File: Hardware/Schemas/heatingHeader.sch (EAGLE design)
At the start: 26 parts, among them IC1 DS1820

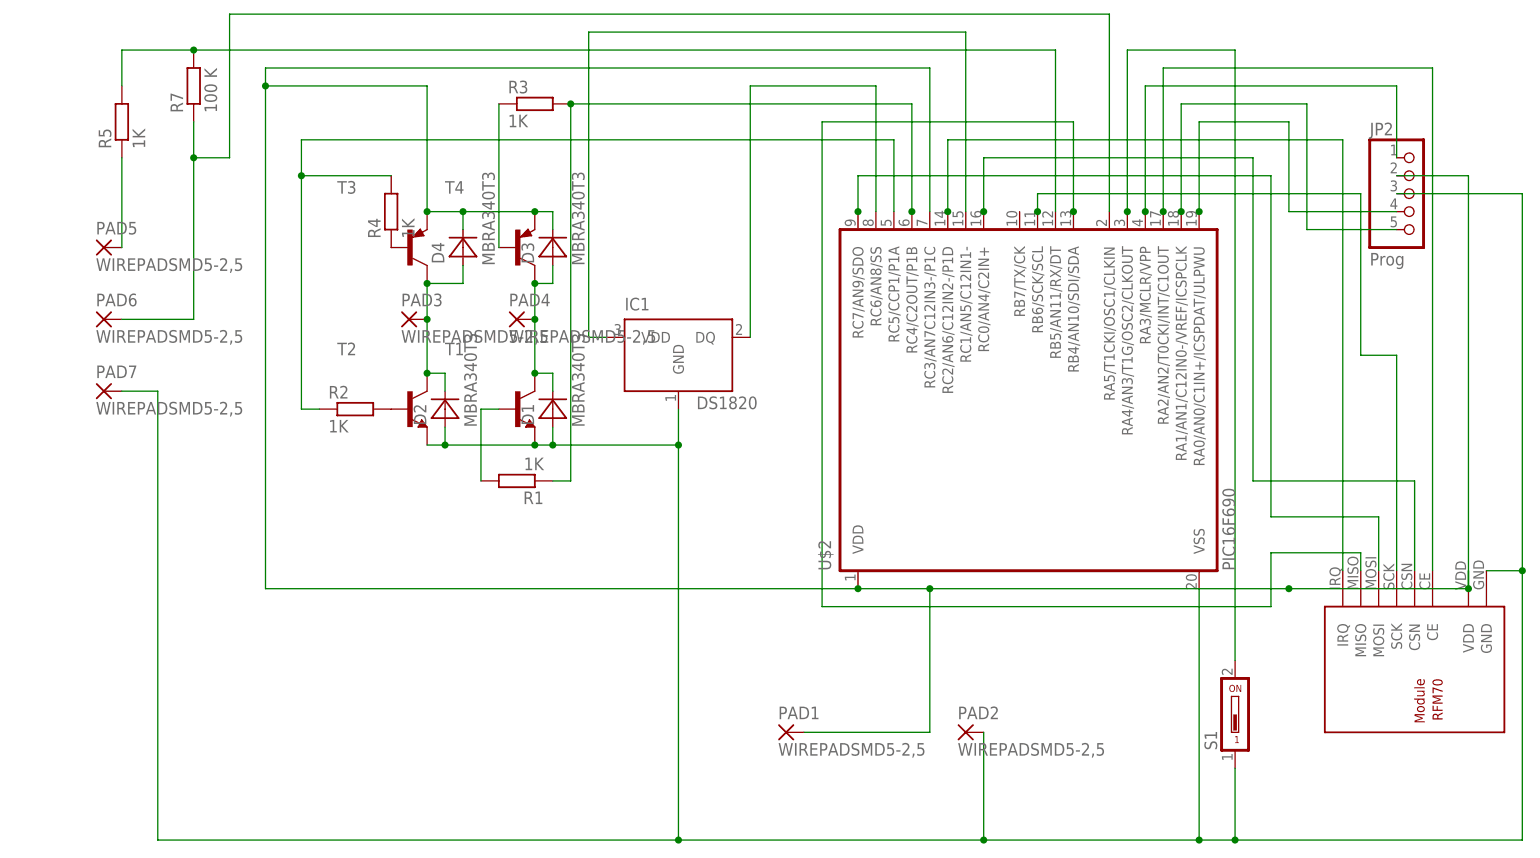
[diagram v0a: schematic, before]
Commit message: a
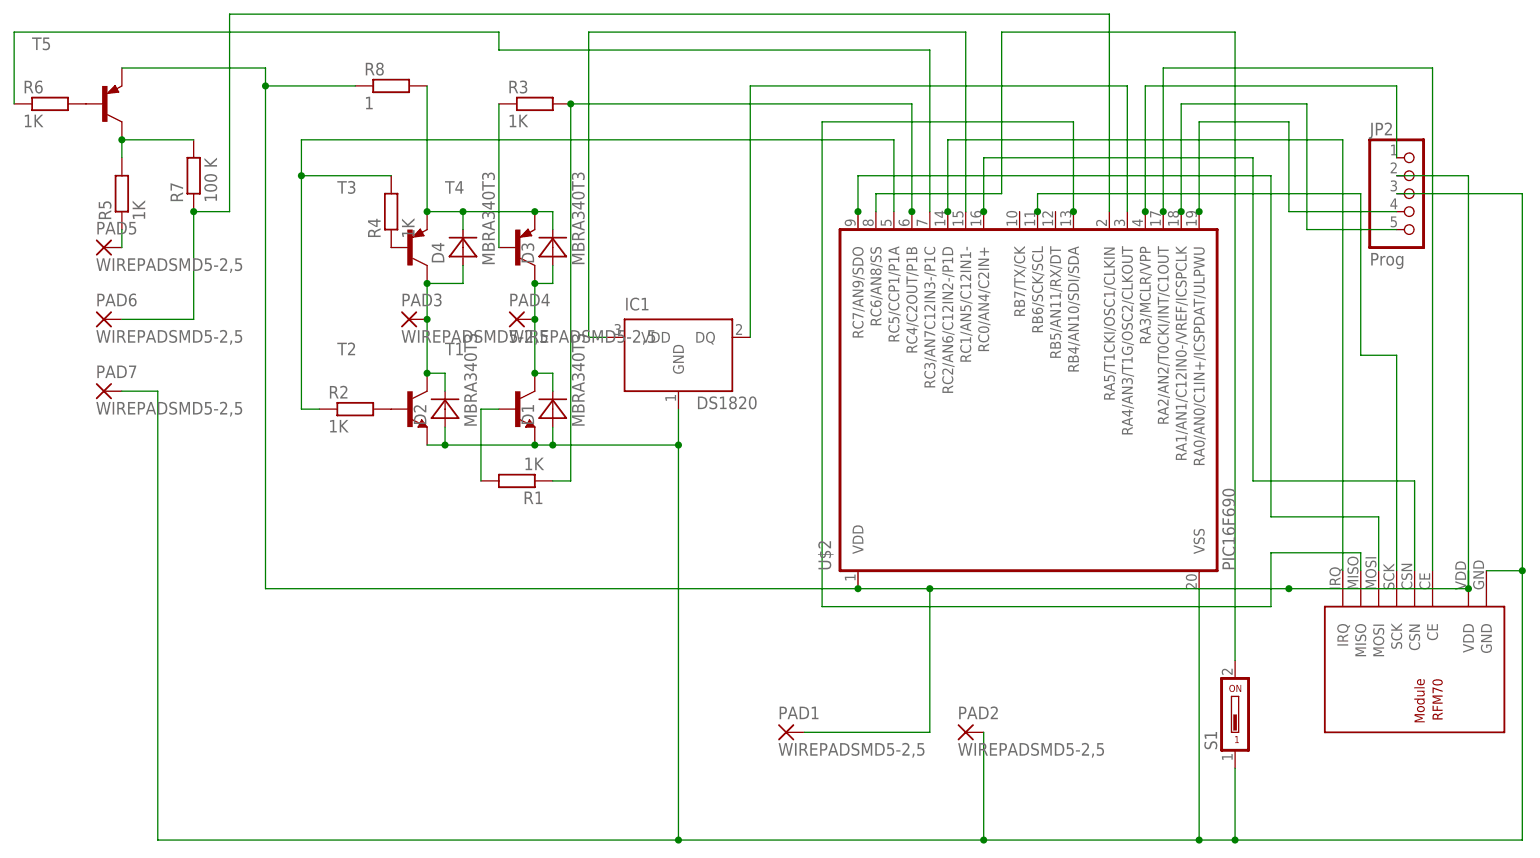
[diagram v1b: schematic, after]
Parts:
- added R6: 1K, resistor:R-EU_R1206
- added R8: 1, resistor:R-EU_R0805W
- added T5: (no value), transistor:BC807-16-PNP-SOT23-BEC
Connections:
- new net N$11: R6.2, T5.B
- new net N$12: R6.1, U$2.RC3/AN7C12IN3-/P1C
- new net N$15: D3.C, D4.C, R8.2, T3.E, T4.E
- net N$1: now also U$2.RA4/AN3/T1G/OSC2/CLKOUT; no longer U$2.RC6/AN8/SS
- net N$10: now also U$2.RC6/AN8/SS; no longer U$2.RA4/AN3/T1G/OSC2/CLKOUT
- net N$2: now also R8.1, T5.E; no longer D3.C, D4.C, T3.E, T4.E, U$2.RC3/AN7C12IN3-/P1C
- net N$28: now also T5.C; no longer U$2.RB5/AN11/RX/DT
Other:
- moved on the sheet: R5, R7
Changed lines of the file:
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@@
 <part name="R7" library="resistor" deviceset="R-EU_" device="R1206" value="100 K"/>
 <part name="S1" library="switch-dil" deviceset="SD4-01" device=""/>
+<part name="T5" library="transistor" deviceset="*-PNP-" device="SOT23-BEC" technology="BC807-16"/>
+<part name="R6" library="resistor" deviceset="R-EU_" device="R1206" value="1K"/>
+<part name="R8" library="resistor" deviceset="R-EU_" device="R0805W" value="1"/>
 </parts>
 <sheets>
@@
 <instance part="PAD4" gate="G$1" x="35.56" y="104.14"/>
 <instance part="PAD5" gate="G$1" x="-22.86" y="114.3"/>
-<instance part="R5" gate="G$1" x="-20.32" y="132.08" rot="R90"/>
+<instance part="R5" gate="G$1" x="-20.32" y="121.92" rot="R90"/>
 <instance part="PAD6" gate="G$1" x="-22.86" y="104.14"/>
 <instance part="PAD7" gate="G$1" x="-22.86" y="93.98"/>
-<instance part="R7" gate="G$1" x="-10.16" y="137.16" rot="R90"/>
+<instance part="R7" gate="G$1" x="-10.16" y="124.46" rot="R90"/>
 <instance part="S1" gate="1" x="137.16" y="48.26"/>
+<instance part="T5" gate="G$1" x="-22.86" y="134.62"/>
+<instance part="R6" gate="G$1" x="-30.48" y="134.62"/>
+<instance part="R8" gate="G$1" x="17.78" y="137.16"/>
 </instances>
 <busses>
@@
 <segment>
 <pinref part="R5" gate="G$1" pin="2"/>
-<wire x1="111.76" y1="142.24" x2="-10.16" y2="142.24" width="0.1524" layer="91"/>
-<wire x1="-10.16" y1="142.24" x2="-20.32" y2="142.24" width="0.1524" layer="91"/>
-<wire x1="-20.32" y1="142.24" x2="-20.32" y2="137.16" width="0.1524" layer="91"/>
-<pinref part="U$2" gate="G$1" pin="RB5/AN11/RX/DT"/>
-<wire x1="111.76" y1="119.38" x2="111.76" y2="142.24" width="0.1524" layer="91"/>
+<wire x1="-10.16" y1="129.54" x2="-20.32" y2="129.54" width="0.1524" layer="91"/>
+<wire x1="-20.32" y1="129.54" x2="-20.32" y2="127" width="0.1524" layer="91"/>
 <pinref part="R7" gate="G$1" pin="2"/>
-<junction x="-10.16" y="142.24"/>
+<pinref part="T5" gate="G$1" pin="C"/>
+<junction x="-20.32" y="129.54"/>
 </segment>
 </net>
@@
 <pinref part="IC1" gate="G$1" pin="DQ"/>
 <wire x1="68.58" y1="101.6" x2="68.58" y2="137.16" width="0.1524" layer="91"/>
-<pinref part="U$2" gate="G$1" pin="RC6/AN8/SS"/>
-<wire x1="68.58" y1="137.16" x2="86.36" y2="137.16" width="0.1524" layer="91"/>
-<wire x1="86.36" y1="137.16" x2="86.36" y2="119.38" width="0.1524" layer="91"/>
+<pinref part="U$2" gate="G$1" pin="RA4/AN3/T1G/OSC2/CLKOUT"/>
+<wire x1="121.92" y1="119.38" x2="121.92" y2="137.16" width="0.1524" layer="91"/>
+<wire x1="121.92" y1="137.16" x2="68.58" y2="137.16" width="0.1524" layer="91"/>
 </segment>
 </net>
@@
 <pinref part="R5" gate="G$1" pin="1"/>
 <pinref part="PAD5" gate="G$1" pin="P"/>
-<wire x1="-20.32" y1="127" x2="-20.32" y2="114.3" width="0.1524" layer="91"/>
+<wire x1="-20.32" y1="116.84" x2="-20.32" y2="114.3" width="0.1524" layer="91"/>
 </segment>
 </net>
 <net name="N$2" class="0">
 <segment>
-<pinref part="T4" gate="G$1" pin="E"/>
-<pinref part="D3" gate="G$1" pin="C"/>
-<wire x1="40.64" y1="116.84" x2="40.64" y2="119.38" width="0.1524" layer="91"/>
-<wire x1="40.64" y1="119.38" x2="38.1" y2="119.38" width="0.1524" layer="91"/>
-<junction x="38.1" y="119.38"/>
-<wire x1="27.94" y1="119.38" x2="38.1" y2="119.38" width="0.1524" layer="91"/>
-<pinref part="D4" gate="G$1" pin="C"/>
-<wire x1="27.94" y1="116.84" x2="27.94" y2="119.38" width="0.1524" layer="91"/>
-<junction x="27.94" y="119.38"/>
-<pinref part="T3" gate="G$1" pin="E"/>
-<wire x1="22.86" y1="119.38" x2="27.94" y2="119.38" width="0.1524" layer="91"/>
-<junction x="22.86" y="119.38"/>
-<wire x1="22.86" y1="137.16" x2="22.86" y2="119.38" width="0.1524" layer="91"/>
-<wire x1="22.86" y1="137.16" x2="0" y2="137.16" width="0.1524" layer="91"/>
+<wire x1="0" y1="139.7" x2="0" y2="137.16" width="0.1524" layer="91"/>
+<pinref part="U$2" gate="G$1" pin="VDD"/>
 <wire x1="0" y1="137.16" x2="0" y2="66.04" width="0.1524" layer="91"/>
-<pinref part="U$2" gate="G$1" pin="RC3/AN7C12IN3-/P1C"/>
-<wire x1="93.98" y1="119.38" x2="93.98" y2="139.7" width="0.1524" layer="91"/>
-<wire x1="93.98" y1="139.7" x2="0" y2="139.7" width="0.1524" layer="91"/>
-<wire x1="0" y1="139.7" x2="0" y2="137.16" width="0.1524" layer="91"/>
-<junction x="0" y="137.16"/>
-<pinref part="U$2" gate="G$1" pin="VDD"/>
 <wire x1="83.82" y1="66.04" x2="93.98" y2="66.04" width="0.1524" layer="91"/>
 <pinref part="U$1" gate="G$1" pin="VDD"/>
@@
 <wire x1="0" y1="66.04" x2="83.82" y2="66.04" width="0.1524" layer="91"/>
 <junction x="83.82" y="66.04"/>
+<pinref part="T5" gate="G$1" pin="E"/>
+<wire x1="-20.32" y1="139.7" x2="0" y2="139.7" width="0.1524" layer="91"/>
+<pinref part="R8" gate="G$1" pin="1"/>
+<wire x1="0" y1="137.16" x2="12.7" y2="137.16" width="0.1524" layer="91"/>
+<junction x="0" y="137.16"/>
 </segment>
 </net>
@@
 <wire x1="119.38" y1="119.38" x2="119.38" y2="147.32" width="0.1524" layer="91"/>
 <wire x1="119.38" y1="147.32" x2="-5.08" y2="147.32" width="0.1524" layer="91"/>
-<wire x1="-5.08" y1="147.32" x2="-5.08" y2="127" width="0.1524" layer="91"/>
+<wire x1="-5.08" y1="147.32" x2="-5.08" y2="119.38" width="0.1524" layer="91"/>
 <pinref part="R7" gate="G$1" pin="1"/>
-<wire x1="-10.16" y1="132.08" x2="-10.16" y2="127" width="0.1524" layer="91"/>
 <pinref part="PAD6" gate="G$1" pin="P"/>
-<wire x1="-10.16" y1="127" x2="-10.16" y2="104.14" width="0.1524" layer="91"/>
+<wire x1="-10.16" y1="119.38" x2="-10.16" y2="104.14" width="0.1524" layer="91"/>
 <wire x1="-10.16" y1="104.14" x2="-20.32" y2="104.14" width="0.1524" layer="91"/>
-<wire x1="-5.08" y1="127" x2="-10.16" y2="127" width="0.1524" layer="91"/>
-<junction x="-10.16" y="127"/>
+<wire x1="-5.08" y1="119.38" x2="-10.16" y2="119.38" width="0.1524" layer="91"/>
+<junction x="-10.16" y="119.38"/>
 </segment>
 </net>
@@
 <segment>
 <pinref part="S1" gate="1" pin="2"/>
-<wire x1="137.16" y1="55.88" x2="137.16" y2="142.24" width="0.1524" layer="91"/>
-<pinref part="U$2" gate="G$1" pin="RA4/AN3/T1G/OSC2/CLKOUT"/>
-<wire x1="137.16" y1="142.24" x2="121.92" y2="142.24" width="0.1524" layer="91"/>
-<wire x1="121.92" y1="142.24" x2="121.92" y2="119.38" width="0.1524" layer="91"/>
-<junction x="121.92" y="119.38"/>
-</segment>
-</net>
+<wire x1="137.16" y1="55.88" x2="137.16" y2="144.78" width="0.1524" layer="91"/>
+<pinref part="U$2" gate="G$1" pin="RC6/AN8/SS"/>
+<wire x1="86.36" y1="119.38" x2="86.36" y2="121.92" width="0.1524" layer="91"/>
+<wire x1="86.36" y1="121.92" x2="104.14" y2="121.92" width="0.1524" layer="91"/>
+<wire x1="104.14" y1="121.92" x2="104.14" y2="144.78" width="0.1524" layer="91"/>
+<wire x1="104.14" y1="144.78" x2="137.16" y2="144.78" width="0.1524" layer="91"/>
+</segment>
+</net>
+<net name="N$11" class="0">
+<segment>
+<pinref part="T5" gate="G$1" pin="B"/>
+<pinref part="R6" gate="G$1" pin="2"/>
+</segment>
+</net>
+<net name="N$12" class="0">
+<segment>
+<pinref part="R6" gate="G$1" pin="1"/>
+<wire x1="-35.56" y1="134.62" x2="-35.56" y2="144.78" width="0.1524" layer="91"/>
+<wire x1="-35.56" y1="144.78" x2="33.02" y2="144.78" width="0.1524" layer="91"/>
+<wire x1="33.02" y1="144.78" x2="33.02" y2="142.24" width="0.1524" layer="91"/>
+<pinref part="U$2" gate="G$1" pin="RC3/AN7C12IN3-/P1C"/>
+<wire x1="33.02" y1="142.24" x2="93.98" y2="142.24" width="0.1524" layer="91"/>
+<wire x1="93.98" y1="142.24" x2="93.98" y2="119.38" width="0.1524" layer="91"/>
+</segment>
+</net>
+<net name="N$15" class="0">
+<segment>
+<pinref part="T4" gate="G$1" pin="E"/>
+<pinref part="D3" gate="G$1" pin="C"/>
+<wire x1="40.64" y1="116.84" x2="40.64" y2="119.38" width="0.1524" layer="91"/>
+<wire x1="40.64" y1="119.38" x2="38.1" y2="119.38" width="0.1524" layer="91"/>
+<junction x="38.1" y="119.38"/>
+<wire x1="27.94" y1="119.38" x2="38.1" y2="119.38" width="0.1524" layer="91"/>
+<pinref part="D4" gate="G$1" pin="C"/>
+<wire x1="27.94" y1="116.84" x2="27.94" y2="119.38" width="0.1524" layer="91"/>
+<junction x="27.94" y="119.38"/>
+<pinref part="T3" gate="G$1" pin="E"/>
+<wire x1="22.86" y1="119.38" x2="27.94" y2="119.38" width="0.1524" layer="91"/>
+<junction x="22.86" y="119.38"/>
+<wire x1="22.86" y1="137.16" x2="22.86" y2="119.38" width="0.1524" layer="91"/>
+<pinref part="R8" gate="G$1" pin="2"/>
+</segment>
+</net>
